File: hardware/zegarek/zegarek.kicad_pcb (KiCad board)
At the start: 2 copper layers, 123.5 x 51 mm, 14 parts, among them J1 Conn_01x02_Socket, J2 Conn_01x02_Pin, Q1 IRF740, U1 MC34063AD

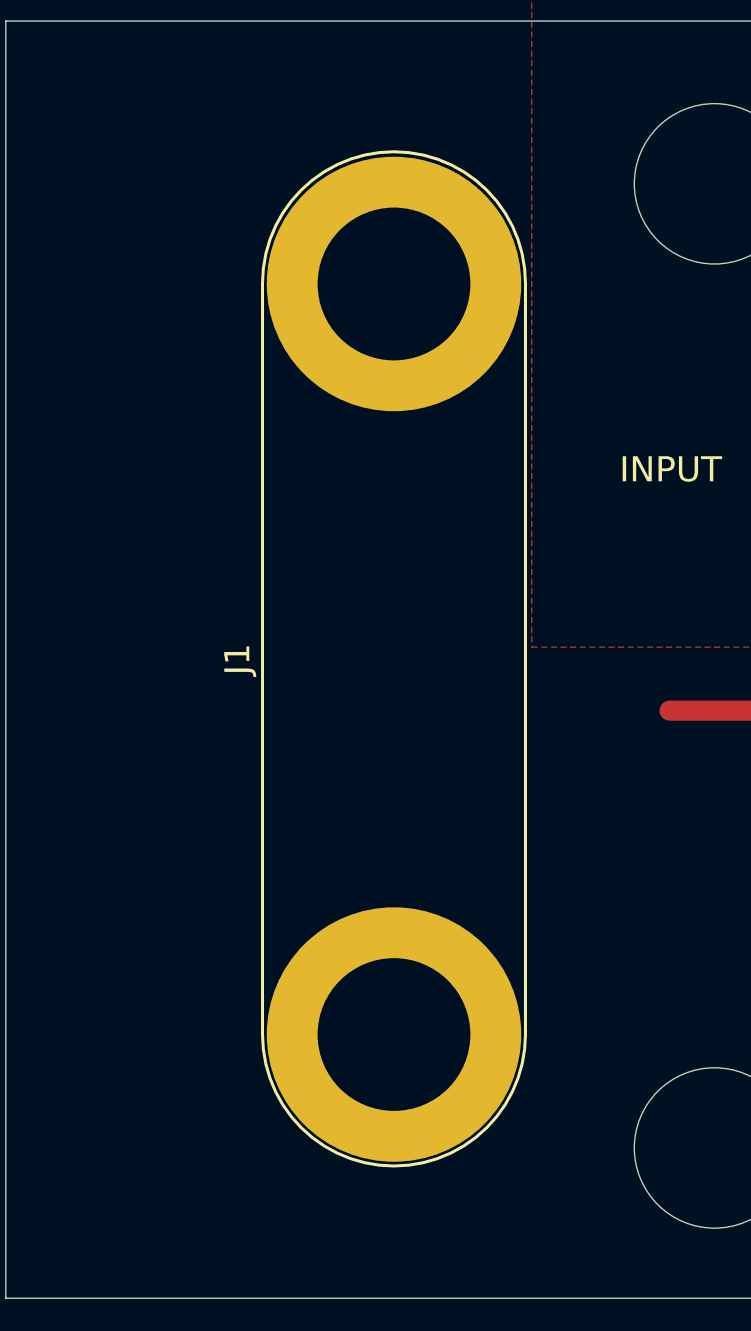
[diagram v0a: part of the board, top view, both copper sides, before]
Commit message: w3
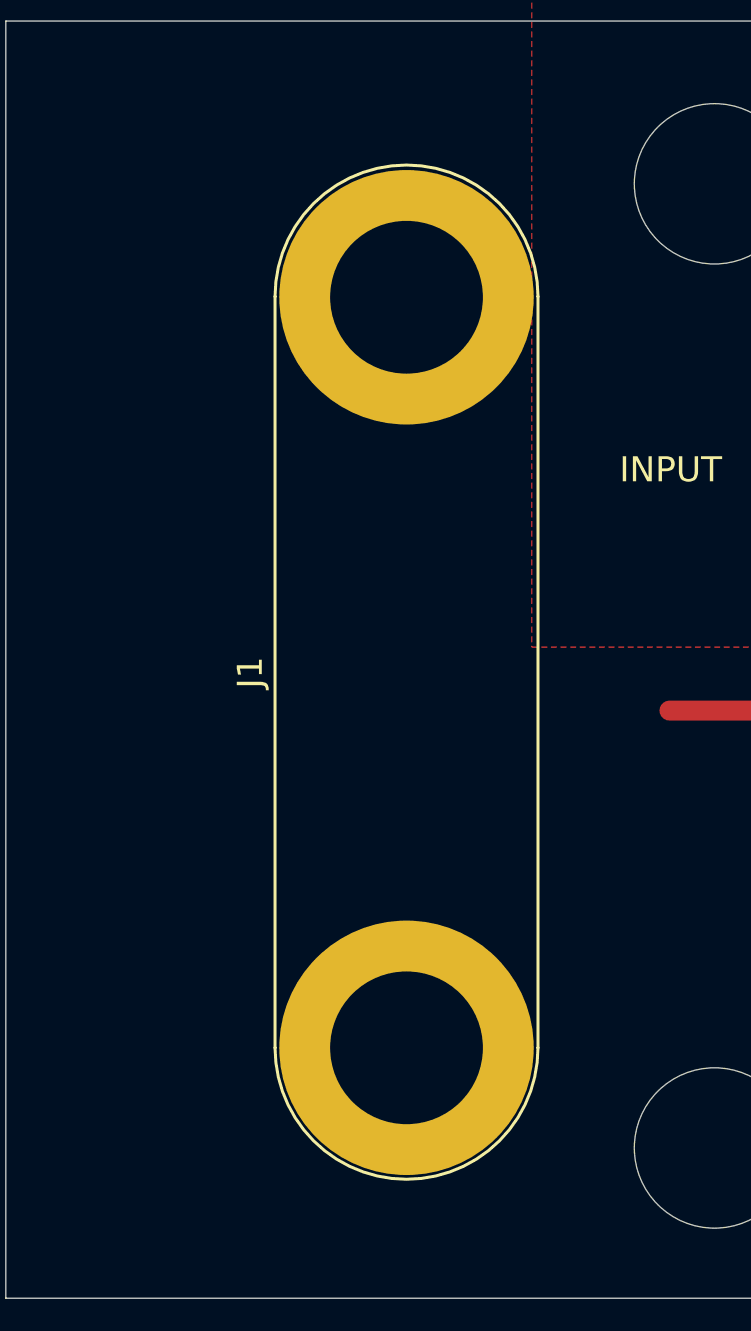
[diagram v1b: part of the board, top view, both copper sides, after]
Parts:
- moved J1 0.73 mm to (108.5, 115.5)
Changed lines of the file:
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@@
 	(footprint "Connector:Banana_Jack_2Pin"
 		(layer "F.Cu")
-		(at 108 114.97 90)
+		(at 108.5 115.5 90)
 		(descr "Dual banana socket, footprint - 2 x 6mm drills")
 		(tags "banana socket")
